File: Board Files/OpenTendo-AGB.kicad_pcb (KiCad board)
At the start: 2 copper layers, 131.3 x 72.4 mm, 221 parts, among them P1 CART-SLOT, P2 LCD, U2 AGB-SRAM, U3 AGB-REG, X2 Crystal

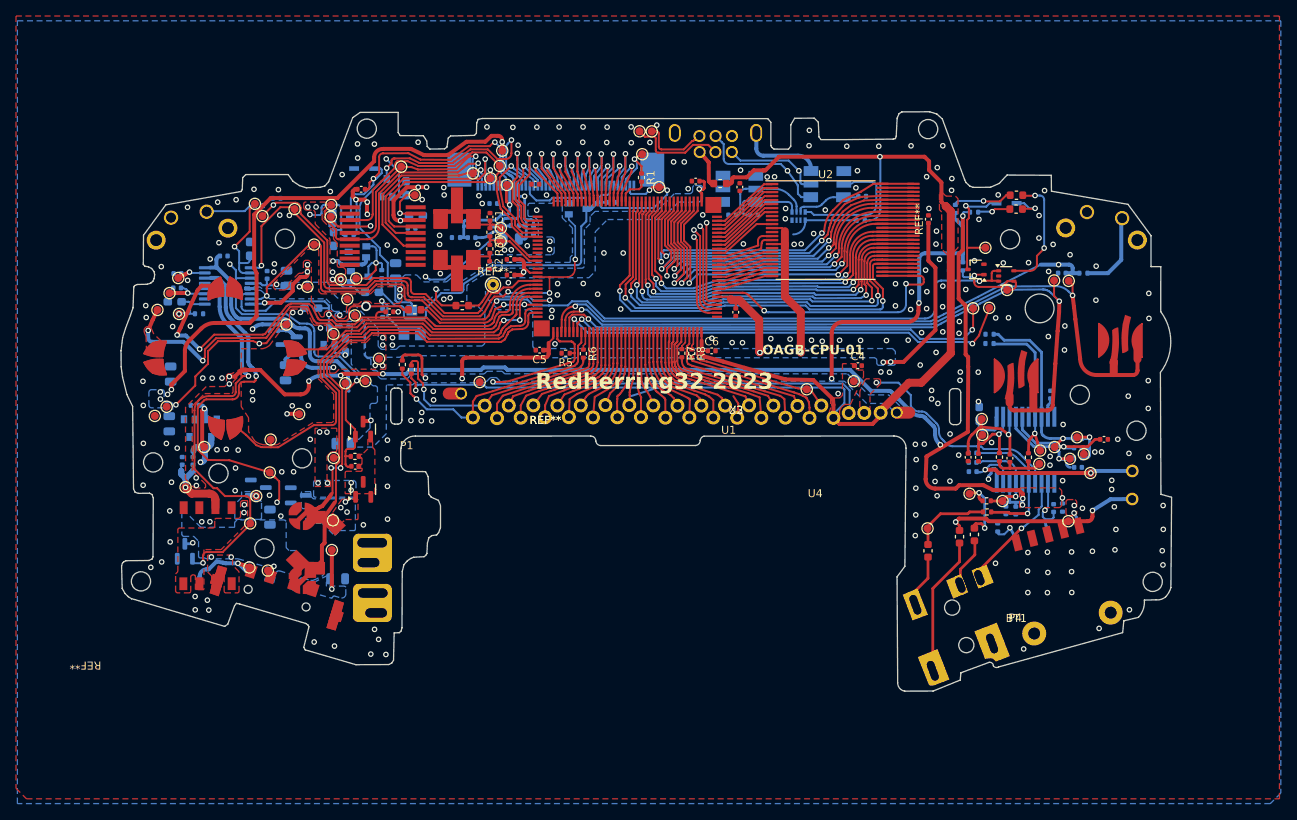
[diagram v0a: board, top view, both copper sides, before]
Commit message: Add files via upload
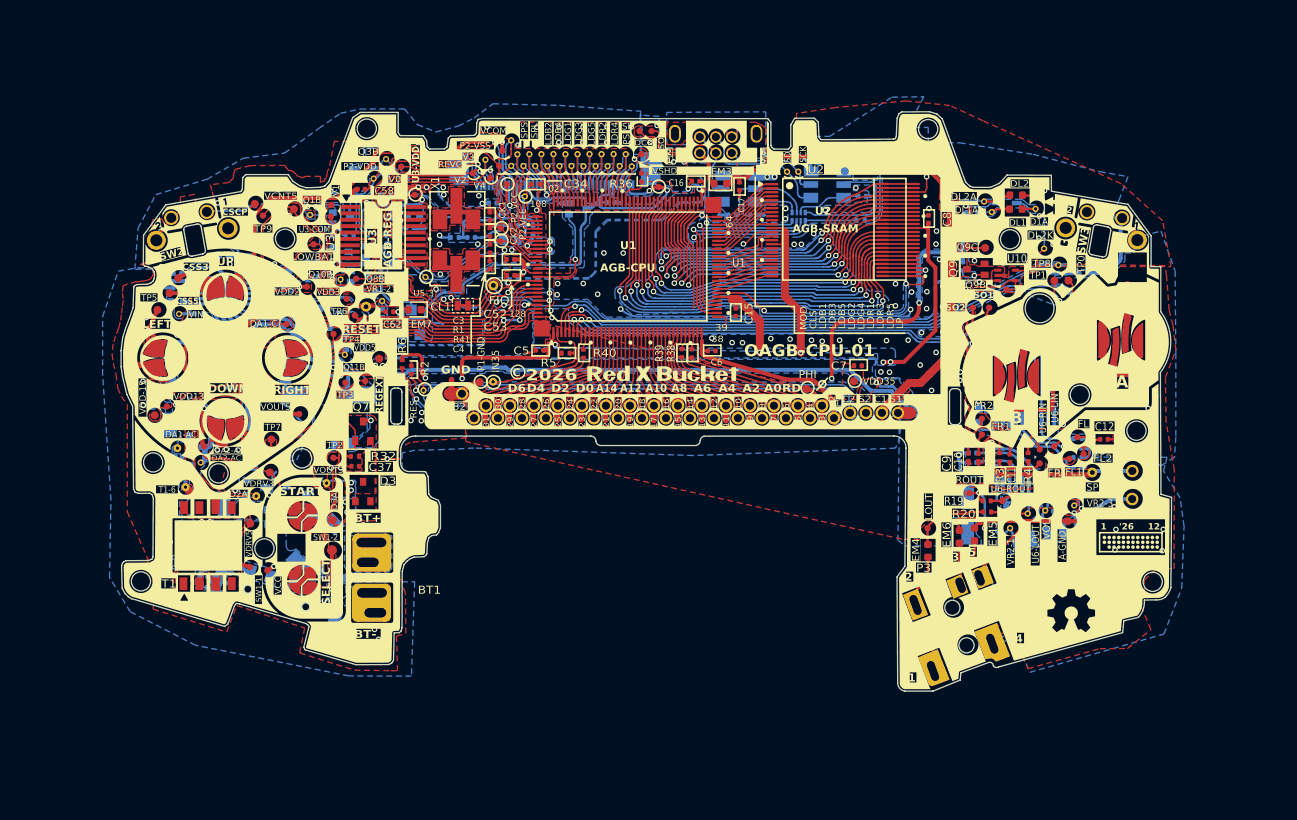
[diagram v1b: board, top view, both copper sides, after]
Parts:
- removed  : SOT-23-Small, OpenTendo-AGB:SOT-23-Small
- removed  : LR, OpenTendo-AGB:LR
- removed  : R_0402_1005Metric, Resistor_SMD:R_0402_1005Metric
- removed  : TestPoint_Pad_D1.0mm, TestPoint:TestPoint_Pad_D1.0mm (x3)
- removed the C1 at (45.9, -59.6)
- removed the C2 at (45.9, -53.6)
- removed the R3 at (45.9, -55.6)
- removed REF**: C_0603_1608Metric_Pad1.08x0.95mm_HandSolder, Capacitor_SMD:C_0603_1608Metric_Pad1.08x0.95mm_HandSolder
- removed REF** (x2): C_0402_1005Metric, Capacitor_SMD:C_0402_1005Metric
- added C13: 0.1u, OpenTendo-AGB:C_0402_1005Metric, B.Cu at (46.2, -61.4)
- added C3: 27p, OpenTendo-AGB:C_0402_1005Metric, F.Cu at (45.9, -59.7)
- added C4: 33p, OpenTendo-AGB:C_0402_1005Metric, F.Cu at (45.9, -53.6)
- added C42: 1u, OpenTendo-AGB:C_0603_1608Metric, B.Cu at (35.4, -63.5)
- added C49: 100p, OpenTendo-AGB:C_0402_1005Metric, B.Cu at (119.3, -28.3)
- added CP1: 100u, OpenTendo-AGB:CP_Elec_5x5.3, B.Cu at (12.7, -21.3)
- added CP2: 100u, OpenTendo-AGB:C_Elec_6.3x5.8, B.Cu at (16.1, -32.1)
- added CP3: 470u, OpenTendo-AGB:C_Elec_8x10.2, B.Cu at (25.9, -37.4)
- added CP4: 100u, OpenTendo-AGB:CP_Elec_5x5.3, B.Cu at (105.6, -22.4)
- added G***: LOGO, LOGO, F.Cu at (67.6, -40.1)
- added G***: LOGO, LOGO, F.Cu at (118.5, -10.4)
- added Q3: DTC114Y, OpenTendo-AGB:SOT-323, B.Cu at (32.9, -63.6)
- added R4: 47k, OpenTendo-AGB:R_0402_1005Metric, F.Cu at (113.2, -29.6)
- added R41: 2.2k, OpenTendo-AGB:R_0402_1005Metric, F.Cu at (45.9, -55.7)
- added SW2: SW_Push, OpenTendo-AGB:L, F.Cu at (10.5, -60.3)
- added TP0: TP0, OpenTendo-AGB:TestPoint_Pad_D1.0mm, F.Cu at (118.2, -51.7)
- added TP10: VOUT3, OpenTendo-AGB:TestPoint_Pad_D1.0mm_VIA, F.Cu at (25.5, -26.4)
- added TP106: VOL, OpenTendo-AGB:TestPoint_Pad_D0.8mm_VIA, F.Cu at (115.3, -22.9)
- added TP107: VR2-3, OpenTendo-AGB:TestPoint_Pad_D0.8mm_VIA, F.Cu at (118.9, -23.6)
- added TP108: VR2-1, OpenTendo-AGB:TestPoint_Pad_D0.8mm_VIA, F.Cu at (110.9, -20.7)
- added TP109: LOUT, OpenTendo-AGB:TestPoint_Pad_D0.8mm, F.Cu at (100.6, -20.7)
- added TP111: SP, OpenTendo-AGB:TestPoint_Pad_D1.25mm_VIA, F.Cu at (121.2, -27.7)
- added TP15: ~{RESET}, OpenTendo-AGB:TestPoint_Pad_D1.25mm_VIA, F.Cu at (30.4, -48.4)
- added TP18: DA2-AC, OpenTendo-AGB:TestPoint_Pad_D0.8mm_VIA, F.Cu at (9.74, -28.9)
- added TP19: DA1-AC, OpenTendo-AGB:TestPoint_Pad_D1.0mm_VIA, F.Cu at (6.83, -30.8)
- added TP28: LOWBAT, OpenTendo-AGB:TestPoint_Pad_D0.8mm, F.Cu at (23.9, -56.2)
- added TP29: DL2A, OpenTendo-AGB:TestPoint_Pad_D0.8mm_VIA, F.Cu at (107.7, -61.6)
- added TP30: DL2K, OpenTendo-AGB:TestPoint_Pad_D0.8mm_VIA, F.Cu at (115.2, -55.7)
- added TP31: DL1A, OpenTendo-AGB:TestPoint_Pad_D0.8mm_VIA, F.Cu at (108.6, -60.3)
- added TP32: D1A, OpenTendo-AGB:TestPoint_Pad_D0.8mm_VIA, F.Cu at (114.1, -60.6)
- added TP35: Q11B, OpenTendo-AGB:TestPoint_Pad_D0.8mm_VIA, F.Cu at (27.8, -42.4)
- added TP36: MOD, OpenTendo-AGB:TestPoint_Pad_D0.8mm_VIA, F.Cu at (48.5, -66.0)
- added TP37: SPS, OpenTendo-AGB:TestPoint_Pad_D0.8mm_VIA, F.Cu at (49.3, -67.5)
- added TP38: CLS, OpenTendo-AGB:TestPoint_Pad_D0.8mm_VIA, F.Cu at (50.1, -66.0)
- added TP39: SPL, OpenTendo-AGB:TestPoint_Pad_D0.8mm_VIA, F.Cu at (50.8, -67.5)
- added TP40: LDB1, OpenTendo-AGB:TestPoint_Pad_D0.8mm_VIA, F.Cu at (51.6, -66.0)
- added TP41: LDB2, OpenTendo-AGB:TestPoint_Pad_D0.8mm_VIA, F.Cu at (52.3, -67.5)
- added TP42: LDB3, OpenTendo-AGB:TestPoint_Pad_D0.8mm_VIA, F.Cu at (53.1, -66.0)
- added TP43: LDB4, OpenTendo-AGB:TestPoint_Pad_D0.8mm_VIA, F.Cu at (53.8, -67.5)
- added TP44: LDB5, OpenTendo-AGB:TestPoint_Pad_D0.8mm_VIA, F.Cu at (54.6, -66.0)
- added TP45: LDG1, OpenTendo-AGB:TestPoint_Pad_D0.8mm_VIA, F.Cu at (55.3, -67.5)
- added TP46: LDG2, OpenTendo-AGB:TestPoint_Pad_D0.8mm_VIA, F.Cu at (56.1, -66.0)
- added TP47: LDG3, OpenTendo-AGB:TestPoint_Pad_D0.8mm_VIA, F.Cu at (56.8, -67.5)
- added TP48: LDG4, OpenTendo-AGB:TestPoint_Pad_D0.8mm_VIA, F.Cu at (57.6, -66.0)
- added TP49: LDG5, OpenTendo-AGB:TestPoint_Pad_D0.8mm_VIA, F.Cu at (58.3, -67.5)
- added TP50: LDR1, OpenTendo-AGB:TestPoint_Pad_D0.8mm_VIA, F.Cu at (59.1, -66.0)
- added TP51: LDR2, OpenTendo-AGB:TestPoint_Pad_D0.8mm_VIA, F.Cu at (59.8, -67.5)
- added TP52: LDR3, OpenTendo-AGB:TestPoint_Pad_D0.8mm_VIA, F.Cu at (60.6, -66.0)
- added TP53: LDR4, OpenTendo-AGB:TestPoint_Pad_D0.8mm_VIA, F.Cu at (61.4, -67.5)
- added TP54: LDR5, OpenTendo-AGB:TestPoint_Pad_D0.8mm_VIA, F.Cu at (62.1, -66.0)
- added TP55: PS, OpenTendo-AGB:TestPoint_Pad_D0.8mm_VIA, F.Cu at (62.9, -67.5)
- added TP56: LP, OpenTendo-AGB:TestPoint_Pad_D0.8mm_VIA, F.Cu at (63.6, -66.0)
- added TP60: P2-VDD, OpenTendo-AGB:TestPoint_Pad_D0.8mm_VIA, F.Cu at (31.4, -64.4)
- added TP61: P2-VEE, OpenTendo-AGB:TestPoint_Pad_D0.8mm_VIA, F.Cu at (50.2, -62.2)
- added TP67: V3, OpenTendo-AGB:TestPoint_Pad_D0.8mm_VIA, F.Cu at (45.3, -66.8)
- added TP70: VCOM, OpenTendo-AGB:TestPoint_Pad_D0.8mm_VIA, F.Cu at (48.5, -69.2)
- added TP71: VR1-2, OpenTendo-AGB:TestPoint_Pad_D0.8mm_VIA, F.Cu at (32.4, -49.1)
- added TP72: U5-3, OpenTendo-AGB:TestPoint_Pad_D0.8mm_VIA, F.Cu at (37.8, -52.1)
- added TP73: Q3B, OpenTendo-AGB:TestPoint_Pad_D0.8mm_VIA, F.Cu at (32.9, -66.9)
- added TP74: Q1B, OpenTendo-AGB:TestPoint_Pad_D0.8mm_VIA, F.Cu at (23.4, -59.9)
- added TP75: IN35, OpenTendo-AGB:TestPoint_Pad_D1.0mm_VIA, F.Cu at (46.3, -39.0)
- added TP78: RES, OpenTendo-AGB:TestPoint_Pad_D0.8mm_VIA, F.Cu at (37.6, -38.0)
- added TP8: TP8, OpenTendo-AGB:TestPoint_Pad_D0.8mm_VIA, F.Cu at (116.9, -53.6)
- added TP93: SD, OpenTendo-AGB:TestPoint_Pad_D0.8mm_VIA, F.Cu at (83.0, -65.3)
- added TP95: SCK, OpenTendo-AGB:TestPoint_Pad_D0.8mm_VIA, F.Cu at (84.4, -65.3)
- added U5: ~, OpenTendo-AGB:SOT-363_SC-70-6, B.Cu at (32.9, -58.5)
- C1, C63, C64: renamed from REF**; value C_0402_1005Metric -> 0.01u; footprint Capacitor_SMD:C_0402_1005Metric -> OpenTendo-AGB:C_0402_1005Metric
- C10: renamed from  ; value C_0402_1005Metric -> 100p; footprint Capacitor_SMD:C_0402_1005Metric -> OpenTendo-AGB:C_0402_1005Metric
- C11: renamed from  ; value C_0402_1005Metric -> 470p; footprint Capacitor_SMD:C_0402_1005Metric -> OpenTendo-AGB:C_0402_1005Metric
- C12, C9: renamed from  ; value C_0402_1005Metric -> 1000p; footprint Capacitor_SMD:C_0402_1005Metric -> OpenTendo-AGB:C_0402_1005Metric
- C14, C22, C23, C26, C32, C39, C40, C41, C45, C46, C47, C50, C51, C55, C59, C8: renamed from REF**; value C_0402_1005Metric -> 0.1u; footprint Capacitor_SMD:C_0402_1005Metric -> OpenTendo-AGB:C_0402_1005Metric
- C15, C16, C17, C34, C52, C53, C58: renamed from  ; value C_0402_1005Metric -> 0.1u; footprint Capacitor_SMD:C_0402_1005Metric -> OpenTendo-AGB:C_0402_1005Metric
- C18, C19, C20: renamed from REF**; value C_0402_1005Metric -> 100p; footprint Capacitor_SMD:C_0402_1005Metric -> OpenTendo-AGB:C_0402_1005Metric
- C2, C24, C28, C30, C38, C57, C61: renamed from REF**; value C_0603_1608Metric_Pad1.08x0.95mm_HandSolder -> 1u; footprint Capacitor_SMD:C_0603_1608Metric_Pad1.08x0.95mm_HandSolder -> OpenTendo-AGB:C_0603_1608Metric
- C25: renamed from REF**; value C_0603_1608Metric_Pad1.08x0.95mm_HandSolder -> 0.47u; footprint Capacitor_SMD:C_0603_1608Metric_Pad1.08x0.95mm_HandSolder -> OpenTendo-AGB:C_0603_1608Metric
- C27, C43, C54: renamed from REF**; value C_0805_2012Metric -> 4.7u; footprint Capacitor_SMD:C_0805_2012Metric -> OpenTendo-AGB:C_0805_2012Metric
- C33, C35, C36: renamed from REF**; value C_0805_2012Metric -> 1u; footprint Capacitor_SMD:C_0805_2012Metric -> OpenTendo-AGB:C_0805_2012Metric
- C37, C62: renamed from  ; value C_0402_1005Metric -> 0.01u; footprint Capacitor_SMD:C_0402_1005Metric -> OpenTendo-AGB:C_0402_1005Metric
- C44, C56: renamed from REF**; value C_0805_2012Metric -> 2.2u; footprint Capacitor_SMD:C_0805_2012Metric -> OpenTendo-AGB:C_0805_2012Metric
- C48: renamed from REF**; value C_0402_1005Metric -> 470p; footprint Capacitor_SMD:C_0402_1005Metric -> OpenTendo-AGB:C_0402_1005Metric
- C5, C6: value C_Small -> 0.1u; footprint Capacitor_SMD:C_0402_1005Metric -> OpenTendo-AGB:C_0402_1005Metric
- C7: renamed from C4; value C_Small -> 0.1u; footprint Capacitor_SMD:C_0402_1005Metric -> OpenTendo-AGB:C_0402_1005Metric
- CL1: renamed from  ; value L_0603_1608Metric -> SolderJumper_2_Bridged; footprint Inductor_SMD:L_0603_1608Metric -> OpenTendo-AGB:Jumper-Bridged
- D1: renamed from REF**; value Diode -> MA112
- D2: renamed from  ; value SOT-23 -> RB411D; footprint Package_TO_SOT_SMD:SOT-23 -> OpenTendo-AGB:SOT-23
- D3: renamed from  ; value SOT-23 -> RB491D; footprint Package_TO_SOT_SMD:SOT-23 -> OpenTendo-AGB:SOT-23
- D4: renamed from REF**; value Diode -> ISS355
- DA1, DA2: renamed from  ; value SOT-23-Small -> DA204U; footprint OpenTendo-AGB:SOT-23-Small -> OpenTendo-AGB:SOT-323
- DL1: renamed from  ; value L_0603_1608Metric -> SML311UT; footprint Inductor_SMD:L_0603_1608Metric -> OpenTendo-AGB:LED_0603_1608Metric
- DL2: renamed from  ; value L_0603_1608Metric -> SML210MT; footprint Inductor_SMD:L_0603_1608Metric -> OpenTendo-AGB:LED_0603_1608Metric
- DZ1: renamed from REF**; value Diode -> 4.7V
- EM1, EM2: renamed from REF**; value EM -> ACM4532-102-3P
- EM3, EM4, EM5, EM6, EM7: renamed from  ; value L_0603_1608Metric -> L_Small; footprint Inductor_SMD:L_0603_1608Metric -> OpenTendo-AGB:L_0603_1608Metric
- F1: renamed from REF**; value Fuse_0805_2012Metric -> 4341.25; footprint Fuse:Fuse_0805_2012Metric -> OpenTendo-AGB:Fuse_0603_1608Metric
- L1: renamed from REF**; value Inductor -> 100u; moved to B.Cu
- P1: value CART-SLOT -> ~
- P2: value LCD -> ~
- P3: renamed from  ; value Audio-Jack -> PHONE JACK
- P4: value ~ -> AGB-LINK
- Q1: renamed from  ; value SOT-23-Small -> DTA123J; footprint OpenTendo-AGB:SOT-23-Small -> OpenTendo-AGB:SOT-323
- Q10: renamed from  ; value SOT-23-Small -> DTC114Y; footprint OpenTendo-AGB:SOT-23-Small -> OpenTendo-AGB:SOT-323
- Q11: renamed from  ; value SOT-23-Small -> DTA114Y; footprint OpenTendo-AGB:SOT-23-Small -> OpenTendo-AGB:SOT-323
- Q2: renamed from  ; value SOT-23-Small -> DTA114T; footprint OpenTendo-AGB:SOT-23-Small -> OpenTendo-AGB:SOT-323
- Q4, Q5: renamed from  ; value SOT-23 -> FDV303N; footprint Package_TO_SOT_SMD:SOT-23 -> OpenTendo-AGB:SOT-23
- Q6: renamed from  ; value SOT-23 -> 2SK1582; footprint Package_TO_SOT_SMD:SOT-23 -> OpenTendo-AGB:SOT-23
- Q7: renamed from  ; value SOT-23 -> SSM3J01F; footprint Package_TO_SOT_SMD:SOT-23 -> OpenTendo-AGB:SOT-23
- Q8: renamed from  ; value SOT-23-Small -> 2SC4081; footprint OpenTendo-AGB:SOT-23-Small -> OpenTendo-AGB:SOT-323
- Q9: renamed from  ; value SOT-323_SC-70 -> 2SC4081; footprint Package_TO_SOT_SMD:SOT-323_SC-70 -> OpenTendo-AGB:SOT-323
- R1: renamed from R2; value R_Small -> 1.5M; footprint Resistor_SMD:R_0402_1005Metric -> OpenTendo-AGB:R_0402_1005Metric
- R10, R37: renamed from REF**; value R_0402_1005Metric -> 470; footprint Resistor_SMD:R_0402_1005Metric -> OpenTendo-AGB:R_0402_1005Metric
- R11, R12, R13: renamed from REF**; value R_0402_1005Metric -> 150; footprint Resistor_SMD:R_0402_1005Metric -> OpenTendo-AGB:R_0402_1005Metric
- R14: renamed from REF**; value R_0402_1005Metric -> 4.7k; footprint Resistor_SMD:R_0402_1005Metric -> OpenTendo-AGB:R_0402_1005Metric
- R15, R16, R18: renamed from REF**; value R_0402_1005Metric -> 33k; footprint Resistor_SMD:R_0402_1005Metric -> OpenTendo-AGB:R_0402_1005Metric
- R17, R35: renamed from REF**; value R_0402_1005Metric -> 100k; footprint Resistor_SMD:R_0402_1005Metric -> OpenTendo-AGB:R_0402_1005Metric
- R19, R20: renamed from  ; value R_0402_1005Metric -> 15; footprint Resistor_SMD:R_0402_1005Metric -> OpenTendo-AGB:R_0402_1005Metric
- R2: renamed from  ; value R_0402_1005Metric -> 10k; footprint Resistor_SMD:R_0402_1005Metric -> OpenTendo-AGB:R_0402_1005Metric
- R25: renamed from REF**; value R_0402_1005Metric -> 47; footprint Resistor_SMD:R_0402_1005Metric -> OpenTendo-AGB:R_0402_1005Metric
- R26, R34: renamed from REF**; value R_0402_1005Metric -> 15k; footprint Resistor_SMD:R_0402_1005Metric -> OpenTendo-AGB:R_0402_1005Metric
- R27: renamed from REF**; value R_0402_1005Metric -> 200k; footprint Resistor_SMD:R_0402_1005Metric -> OpenTendo-AGB:R_0402_1005Metric
- R28: renamed from REF**; value R_0402_1005Metric -> 56k; footprint Resistor_SMD:R_0402_1005Metric -> OpenTendo-AGB:R_0402_1005Metric
- R29: renamed from REF**; value R_0402_1005Metric -> 18k; footprint Resistor_SMD:R_0402_1005Metric -> OpenTendo-AGB:R_0402_1005Metric
- R3: renamed from  ; value R_0402_1005Metric -> 47k; footprint Resistor_SMD:R_0402_1005Metric -> OpenTendo-AGB:R_0402_1005Metric
- R30, R31, R7, R8: renamed from REF**; value R_0402_1005Metric -> 47k; footprint Resistor_SMD:R_0402_1005Metric -> OpenTendo-AGB:R_0402_1005Metric
- R32: renamed from  ; value R_0402_1005Metric -> 1M; footprint Resistor_SMD:R_0402_1005Metric -> OpenTendo-AGB:R_0402_1005Metric
- R33: renamed from REF**; value R_0402_1005Metric -> 5.1; footprint Resistor_SMD:R_0402_1005Metric -> OpenTendo-AGB:R_0402_1005Metric
- R36: renamed from R1; value R_Small -> 270; footprint Resistor_SMD:R_0402_1005Metric -> OpenTendo-AGB:R_0402_1005Metric
- R38: renamed from R8; value R_Small -> 47; footprint Resistor_SMD:R_0402_1005Metric -> OpenTendo-AGB:R_0402_1005Metric
- R39: renamed from R7; value R_Small -> 47; footprint Resistor_SMD:R_0402_1005Metric -> OpenTendo-AGB:R_0402_1005Metric
- R40: renamed from R6; value R_Small -> 15; footprint Resistor_SMD:R_0402_1005Metric -> OpenTendo-AGB:R_0402_1005Metric
- R43, R44: renamed from REF**; value R_0402_1005Metric -> 15; footprint Resistor_SMD:R_0402_1005Metric -> OpenTendo-AGB:R_0402_1005Metric
- R5: value R_Small -> 100k; footprint Resistor_SMD:R_0402_1005Metric -> OpenTendo-AGB:R_0402_1005Metric
- R6: renamed from  ; value R_0402_1005Metric -> 100k; footprint Resistor_SMD:R_0402_1005Metric -> OpenTendo-AGB:R_0402_1005Metric
- RA1: renamed from REF**; value RA -> 330
- SP1: renamed from  
- SW1: renamed from REF**; value Power Switch -> AGB-SW; moved to B.Cu
- SW3: renamed from  ; value R -> SW_Push
- SW4: renamed from  ; value AB -> ~
- SW5: renamed from  ; value StartSelect -> ~
- T1: renamed from  ; value Coil -> AGB-XFRM
- TP1: renamed from  ; value TestPoint_Pad_D1.0mm -> TP1; footprint TestPoint:TestPoint_Pad_D1.0mm -> OpenTendo-AGB:TestPoint_Pad_D1.0mm
- TP100: renamed from  ; value TestPoint_Pad_D1.0mm -> FL1; footprint TestPoint:TestPoint_Pad_D1.0mm -> OpenTendo-AGB:TestPoint_Pad_D0.8mm
- TP101: renamed from  ; value TestPoint_Pad_D1.0mm -> FL2; footprint TestPoint:TestPoint_Pad_D1.0mm -> OpenTendo-AGB:TestPoint_Pad_D0.8mm
- TP102: renamed from  ; value TestPoint_Pad_D1.0mm -> FR1; footprint TestPoint:TestPoint_Pad_D1.0mm -> OpenTendo-AGB:TestPoint_Pad_D0.8mm
- TP103: renamed from  ; value TestPoint_Pad_D1.0mm -> FR2; footprint TestPoint:TestPoint_Pad_D1.0mm -> OpenTendo-AGB:TestPoint_Pad_D0.8mm
- TP104: renamed from  ; value TestPoint_Pad_D1.0mm -> U6-LOUT; footprint TestPoint:TestPoint_Pad_D1.0mm -> OpenTendo-AGB:TestPoint_Pad_D0.8mm_VIA
- TP105: renamed from  ; value TestPoint_Pad_D1.0mm -> U6-ROUT; footprint TestPoint:TestPoint_Pad_D1.0mm -> OpenTendo-AGB:TestPoint_Pad_D0.8mm
- TP11: renamed from  ; value TestPoint_Pad_D1.0mm -> VDRV3; footprint TestPoint:TestPoint_Pad_D1.0mm -> OpenTendo-AGB:TestPoint_Pad_D1.0mm
- TP110: renamed from  ; value TestPoint_Pad_D1.0mm -> ROUT; footprint TestPoint:TestPoint_Pad_D1.0mm -> OpenTendo-AGB:TestPoint_Pad_D0.8mm
- TP112: renamed from  ; value TestPoint_Pad_D1.0mm -> A-GND; footprint TestPoint:TestPoint_Pad_D1.0mm -> OpenTendo-AGB:TestPoint_Pad_D1.0mm
- TP113: renamed from  ; value TestPoint_Pad_D1.0mm -> VDD3; footprint TestPoint:TestPoint_Pad_D1.0mm -> OpenTendo-AGB:TestPoint_Pad_D0.8mm
- TP114: renamed from  ; value TestPoint_Pad_D1.0mm -> R-OUT; footprint TestPoint:TestPoint_Pad_D1.0mm -> OpenTendo-AGB:TestPoint_Pad_D0.8mm
- TP115: renamed from  ; value TestPoint_Pad_D1.0mm -> L-OUT; footprint TestPoint:TestPoint_Pad_D1.0mm -> OpenTendo-AGB:TestPoint_Pad_D0.8mm
- TP116: renamed from  ; value TestPoint_Pad_D1.0mm -> T1-6; footprint TestPoint:TestPoint_Pad_D1.0mm -> OpenTendo-AGB:TestPoint_Pad_D1.0mm_VIA
- TP12: renamed from  ; value TestPoint_Pad_D1.0mm -> VDD2; footprint TestPoint:TestPoint_Pad_D1.0mm -> OpenTendo-AGB:TestPoint_Pad_D0.8mm
- TP13: renamed from  ; value TestPoint_Pad_D1.0mm -> VDRV5; footprint TestPoint:TestPoint_Pad_D1.0mm -> OpenTendo-AGB:TestPoint_Pad_D1.0mm
- TP14: renamed from  ; value TestPoint_Pad_D1.0mm -> VOUT5; footprint TestPoint:TestPoint_Pad_D1.0mm -> OpenTendo-AGB:TestPoint_Pad_D0.8mm
- TP16: renamed from  ; value TestPoint_Pad_D1.0mm -> D3A; footprint TestPoint:TestPoint_Pad_D1.0mm -> OpenTendo-AGB:TestPoint_Pad_D1.0mm
- TP17: renamed from  ; value TestPoint_Pad_D1.0mm -> D2A; footprint TestPoint:TestPoint_Pad_D1.0mm -> OpenTendo-AGB:TestPoint_Pad_D1.0mm_VIA
- TP2: renamed from  ; value TestPoint_Pad_D1.0mm -> TP2; footprint TestPoint:TestPoint_Pad_D1.0mm -> OpenTendo-AGB:TestPoint_Pad_D0.8mm
- TP20: renamed from  ; value TestPoint_Pad_D1.0mm -> DA2-A; footprint TestPoint:TestPoint_Pad_D1.0mm -> OpenTendo-AGB:TestPoint_Pad_D0.8mm
- TP21: renamed from  ; value TestPoint_Pad_D1.0mm -> DA1-C; footprint TestPoint:TestPoint_Pad_D1.0mm -> OpenTendo-AGB:TestPoint_Pad_D0.8mm
- TP22: renamed from  ; value TestPoint_Pad_D1.0mm -> VDD13; footprint TestPoint:TestPoint_Pad_D1.0mm -> OpenTendo-AGB:TestPoint_Pad_D0.8mm
- TP23: renamed from  ; value TestPoint_Pad_D1.0mm -> VDD-15; footprint TestPoint:TestPoint_Pad_D1.0mm -> OpenTendo-AGB:TestPoint_Pad_D1.0mm
- TP24: renamed from  ; value TestPoint_Pad_D1.0mm -> VDD5; footprint TestPoint:TestPoint_Pad_D1.0mm -> OpenTendo-AGB:TestPoint_Pad_D1.0mm
- TP25: renamed from  ; value TestPoint_Pad_D1.0mm -> Q8B; footprint TestPoint:TestPoint_Pad_D1.0mm -> OpenTendo-AGB:TestPoint_Pad_D0.8mm
- TP26: renamed from  ; value TestPoint_Pad_D1.0mm -> VSHD; footprint TestPoint:TestPoint_Pad_D1.0mm -> OpenTendo-AGB:TestPoint_Pad_D0.8mm
- TP27: renamed from  ; value TestPoint_Pad_D1.0mm -> Q10B; footprint TestPoint:TestPoint_Pad_D1.0mm -> OpenTendo-AGB:TestPoint_Pad_D0.8mm_VIA
- TP3: renamed from  ; value TestPoint_Pad_D1.0mm -> TP3; footprint TestPoint:TestPoint_Pad_D1.0mm -> OpenTendo-AGB:TestPoint_Pad_D0.8mm
- TP33: renamed from  ; value TestPoint_Pad_D1.0mm -> Q9C; footprint TestPoint:TestPoint_Pad_D1.0mm -> OpenTendo-AGB:TestPoint_Pad_D1.0mm
- TP34: renamed from  ; value TestPoint_Pad_D1.0mm -> Q9B; footprint TestPoint:TestPoint_Pad_D1.0mm -> OpenTendo-AGB:TestPoint_Pad_D0.8mm
- TP4: renamed from  ; value TestPoint_Pad_D1.0mm -> TP4; footprint TestPoint:TestPoint_Pad_D1.0mm -> OpenTendo-AGB:TestPoint_Pad_D0.8mm
- TP5: renamed from  ; value TestPoint_Pad_D1.0mm -> TP5; footprint TestPoint:TestPoint_Pad_D1.0mm -> OpenTendo-AGB:TestPoint_Pad_D1.0mm
- TP57: renamed from  ; value TestPoint_Pad_D1.0mm -> DCK; footprint TestPoint:TestPoint_Pad_D1.0mm -> OpenTendo-AGB:TestPoint_Pad_D0.8mm
- TP58: renamed from  ; value TestPoint_Pad_D1.0mm -> P2-VSS; footprint TestPoint:TestPoint_Pad_D1.0mm -> OpenTendo-AGB:TestPoint_Pad_D0.8mm
- TP59: renamed from  ; value TestPoint_Pad_D1.0mm -> P2-VCC; footprint TestPoint:TestPoint_Pad_D1.0mm -> OpenTendo-AGB:TestPoint_Pad_D0.8mm
- TP6: renamed from  ; value TestPoint_Pad_D1.0mm -> TP6; footprint TestPoint:TestPoint_Pad_D1.0mm -> OpenTendo-AGB:TestPoint_Pad_D0.8mm
- TP62: renamed from  ; value TestPoint_Pad_D1.0mm -> REVC; footprint TestPoint:TestPoint_Pad_D1.0mm -> OpenTendo-AGB:TestPoint_Pad_D0.8mm
- TP63: renamed from  ; value TestPoint_Pad_D1.0mm -> U3-VDD; footprint TestPoint:TestPoint_Pad_D1.0mm -> OpenTendo-AGB:TestPoint_Pad_D0.8mm
- TP64: renamed from  ; value TestPoint_Pad_D1.0mm -> V0; footprint TestPoint:TestPoint_Pad_D1.0mm -> OpenTendo-AGB:TestPoint_Pad_D0.8mm
- TP65: renamed from  ; value TestPoint_Pad_D1.0mm -> V1; footprint TestPoint:TestPoint_Pad_D1.0mm -> OpenTendo-AGB:TestPoint_Pad_D0.8mm
- TP66: renamed from  ; value TestPoint_Pad_D1.0mm -> V2; footprint TestPoint:TestPoint_Pad_D1.0mm -> OpenTendo-AGB:TestPoint_Pad_D0.8mm
- TP68: renamed from  ; value TestPoint_Pad_D1.0mm -> V4; footprint TestPoint:TestPoint_Pad_D1.0mm -> OpenTendo-AGB:TestPoint_Pad_D0.8mm
- TP69: renamed from  ; value TestPoint_Pad_D1.0mm -> U3-COM; footprint TestPoint:TestPoint_Pad_D1.0mm -> OpenTendo-AGB:TestPoint_Pad_D0.8mm
- TP7: renamed from  ; value TestPoint_Pad_D1.0mm -> TP7; footprint TestPoint:TestPoint_Pad_D1.0mm -> OpenTendo-AGB:TestPoint_Pad_D1.0mm
- TP76: renamed from  ; value TestPoint_Pad_D1.0mm -> VDD35; footprint TestPoint:TestPoint_Pad_D1.0mm -> OpenTendo-AGB:TestPoint_Pad_D1.0mm
- TP77: renamed from  ; value TestPoint_Pad_D1.0mm -> PHI; footprint TestPoint:TestPoint_Pad_D1.0mm -> OpenTendo-AGB:TestPoint_Pad_D1.0mm
- TP79: renamed from  ; value TestPoint_Pad_D1.0mm -> P1-GND; footprint TestPoint:TestPoint_Pad_D1.0mm -> OpenTendo-AGB:TestPoint_Pad_D1.0mm
- TP80: renamed from  ; value TestPoint_Pad_D1.0mm -> CK1; footprint TestPoint:TestPoint_Pad_D1.0mm -> OpenTendo-AGB:TestPoint_Pad_D0.8mm
- TP81: renamed from  ; value TestPoint_Pad_D1.0mm -> CK2; footprint TestPoint:TestPoint_Pad_D1.0mm -> OpenTendo-AGB:TestPoint_Pad_D0.8mm
- TP82: renamed from REF**; value TestPoint_THTPad_D1.5mm_Drill0.7mm -> FIQ; footprint TestPoint:TestPoint_THTPad_D1.5mm_Drill0.7mm -> OpenTendo-AGB:TestPoint_Pad_D1.25mm_VIA
- TP83: renamed from  ; value TestPoint_Pad_D1.0mm -> SW1-2; footprint TestPoint:TestPoint_Pad_D1.0mm -> OpenTendo-AGB:TestPoint_Pad_D1.25mm
- TP84: renamed from  ; value TestPoint_Pad_D1.0mm -> SW1-1; footprint TestPoint:TestPoint_Pad_D1.0mm -> OpenTendo-AGB:TestPoint_Pad_D0.8mm
- TP85: renamed from  ; value TestPoint_Pad_D1.0mm -> VCC; footprint TestPoint:TestPoint_Pad_D1.0mm -> OpenTendo-AGB:TestPoint_Pad_D0.8mm
- TP86: renamed from  ; value TestPoint_Pad_D1.0mm -> C_SCP; footprint TestPoint:TestPoint_Pad_D1.0mm -> OpenTendo-AGB:TestPoint_Pad_D1.0mm
- TP87: renamed from  ; value TestPoint_Pad_D1.0mm -> C_SS5; footprint TestPoint:TestPoint_Pad_D1.0mm -> OpenTendo-AGB:TestPoint_Pad_D1.0mm
- TP88: renamed from  ; value TestPoint_Pad_D1.0mm -> C_SS3; footprint TestPoint:TestPoint_Pad_D1.0mm -> OpenTendo-AGB:TestPoint_Pad_D1.0mm
- TP89: renamed from  ; value TestPoint_Pad_D1.0mm -> VIN; footprint TestPoint:TestPoint_Pad_D1.0mm -> OpenTendo-AGB:TestPoint_Pad_D0.8mm_VIA
- TP9: renamed from  ; value TestPoint_Pad_D1.0mm -> TP9; footprint TestPoint:TestPoint_Pad_D1.0mm -> OpenTendo-AGB:TestPoint_Pad_D0.8mm
- TP90: renamed from  ; value TestPoint_Pad_D1.0mm -> REG_EXT; footprint TestPoint:TestPoint_Pad_D1.0mm -> OpenTendo-AGB:TestPoint_Pad_D0.8mm
- TP91: renamed from  ; value TestPoint_Pad_D1.0mm -> VCNT5; footprint TestPoint:TestPoint_Pad_D1.0mm -> OpenTendo-AGB:TestPoint_Pad_D1.0mm
- TP92: renamed from  ; value TestPoint_Pad_D1.0mm -> SO; footprint TestPoint:TestPoint_Pad_D1.0mm -> OpenTendo-AGB:TestPoint_Pad_D0.8mm
- TP94: renamed from  ; value TestPoint_Pad_D1.0mm -> SI; footprint TestPoint:TestPoint_Pad_D1.0mm -> OpenTendo-AGB:TestPoint_Pad_D0.8mm
- TP96: renamed from  ; value TestPoint_Pad_D1.0mm -> U6-LIN; footprint TestPoint:TestPoint_Pad_D1.0mm -> OpenTendo-AGB:TestPoint_Pad_D0.8mm
- TP97: renamed from  ; value TestPoint_Pad_D1.0mm -> U6-RIN; footprint TestPoint:TestPoint_Pad_D1.0mm -> OpenTendo-AGB:TestPoint_Pad_D0.8mm
- TP98: renamed from  ; value TestPoint_Pad_D1.0mm -> FL; footprint TestPoint:TestPoint_Pad_D1.0mm -> OpenTendo-AGB:TestPoint_Pad_D0.8mm
- TP99: renamed from  ; value TestPoint_Pad_D1.0mm -> FR; footprint TestPoint:TestPoint_Pad_D1.0mm -> OpenTendo-AGB:TestPoint_Pad_D0.8mm
- U1: value ~ -> AGB-CPU
- U10: renamed from  ; value SOT-353_SC-70-5 -> ~; footprint Package_TO_SOT_SMD:SOT-353_SC-70-5 -> OpenTendo-AGB:SOT-353_SC-70-5
- U2: value AGB-SRAM -> ~
- U4: renamed from REF**; value TSSOP-16_4.4x5mm_P0.65mm -> ~; footprint Package_SO:TSSOP-16_4.4x5mm_P0.65mm -> OpenTendo-AGB:TSSOP-16_4.4x5mm_P0.65mm
- U6: renamed from  ; value AGB-REG -> AGB-AMP; footprint OpenTendo-AGB:AGB-REG -> OpenTendo-AGB:AGB-AMP
- VR1: renamed from  ; value SOT-23-Large -> 50k; footprint OpenTendo-AGB:SOT-23-Large -> OpenTendo-AGB:VR1
- VR2: renamed from REF**; value Thumbwheel -> 30k; moved to B.Cu
- X1: renamed from X2; value Crystal -> 4.194304MHz
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- renumbered U4 to SW6
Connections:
- net /A renamed /CPU/TP0
- net /B renamed /CPU/TP1
- net /CART-A0 renamed /CPU/A_{0}
- net /CART-A1 renamed /CPU/A_{1}
- net /CART-A10 renamed /CPU/A_{10}
- net /CART-A11 renamed /CPU/A_{11}
- net /CART-A12 renamed /CPU/A_{12}
- net /CART-A13 renamed /CPU/A_{13}
- net /CART-A14 renamed /CPU/A_{14}
- net /CART-A15 renamed /CPU/A_{15}
- net /CART-A2 renamed /CPU/A_{2}
- net /CART-A3 renamed /CPU/A_{3}
- net /CART-A4 renamed /CPU/A_{4}
- net /CART-A5 renamed /CPU/A_{5}
- net /CART-A6 renamed /CPU/A_{6}
- net /CART-A7 renamed /CPU/A_{7}
- net /CART-A8 renamed /CPU/A_{8}
- net /CART-A9 renamed /CPU/A_{9}
- net /CART-D0 renamed /CPU/D_{0}
- net /CART-D1 renamed /CPU/D_{1}
- net /CART-D2 renamed /CPU/D_{2}
- net /CART-D3 renamed /CPU/D_{3}
- net /CART-D4 renamed /CPU/D_{4}
- net /CART-D5 renamed /CPU/D_{5}
- net /CART-D6 renamed /CPU/D_{6}
- net /CART-D7 renamed /CPU/D_{7}
- net /CLK1 renamed /CPU/CK1
- net /CLK2 renamed /CPU/CK2
- net /CLS renamed /CPU/CLS
- net /DCK renamed /CPU/DCK_{R}
- net /DOWN renamed /CPU/TP7
- net /IN35 renamed /CPU/IN35
- net /LDB1 renamed /CPU/LDB1
- net /LDB2 renamed /CPU/LDB2
- net /LDB3 renamed /CPU/LDB3
- net /LDB4 renamed /CPU/LDB4
- net /LDB5 renamed /CPU/LDB5
- net /LDG1 renamed /CPU/LDG1
- net /LDG2 renamed /CPU/LDG2
- net /LDG3 renamed /CPU/LDG3
- net /LDG4 renamed /CPU/LDG4
- net /LDG5 renamed /CPU/LDG5
- net /LDR1 renamed /CPU/LDR1
- net /LDR2 renamed /CPU/LDR2
- net /LDR3 renamed /CPU/LDR3
- net /LDR4 renamed /CPU/LDR4
- net /LDR5 renamed /CPU/LDR5
- net /LEFT renamed /CPU/TP5
- net /LP renamed /CPU/LP
- net /MOD renamed /CPU/MOD
- net /PHI renamed /CPU/PHI
- net /PS renamed /CPU/PS
- net /REVC renamed /CPU/REVC
- net /RIGHT renamed /CPU/TP4
- net /SELECT renamed /CPU/TP2
- net /SPL renamed /CPU/SPL
- net /SPS renamed /CPU/SPS
- net /SRAM-A0 renamed /CPU/MA_{0}
- net /SRAM-A1 renamed /CPU/MA_{1}
- net /SRAM-A10 renamed /CPU/MA_{10}
- net /SRAM-A11 renamed /CPU/MA_{11}
- net /SRAM-A12 renamed /CPU/MA_{12}
- net /SRAM-A13 renamed /CPU/MA_{13}
- net /SRAM-A14 renamed /CPU/MA_{14}
- net /SRAM-A15 renamed /CPU/MA_{15}
- net /SRAM-A16 renamed /CPU/MA_{16}
- net /SRAM-A2 renamed /CPU/MA_{2}
- net /SRAM-A3 renamed /CPU/MA_{3}
- net /SRAM-A4 renamed /CPU/MA_{4}
- net /SRAM-A5 renamed /CPU/MA_{5}
- net /SRAM-A6 renamed /CPU/MA_{6}
- net /SRAM-A8 renamed /CPU/MA_{8}
- net /SRAM-A9 renamed /CPU/MA_{9}
- net /SRAM-I/O1 renamed /CPU/MD_{0}
- net /SRAM-I/O10 renamed /CPU/MD_{9}
- net /SRAM-I/O11 renamed /CPU/MD_{10}
- net /SRAM-I/O12 renamed /CPU/MD_{11}
- net /SRAM-I/O13 renamed /CPU/MD_{12}
- net /SRAM-I/O14 renamed /CPU/MD_{13}
- net /SRAM-I/O15 renamed /CPU/MD_{14}
- net /SRAM-I/O16 renamed /CPU/MD_{15}
- net /SRAM-I/O2 renamed /CPU/MD_{1}
- net /SRAM-I/O3 renamed /CPU/MD_{2}
- net /SRAM-I/O4 renamed /CPU/MD_{3}
- net /SRAM-I/O5 renamed /CPU/MD_{4}
- net /SRAM-I/O6 renamed /CPU/MD_{5}
- net /SRAM-I/O7 renamed /CPU/MD_{6}
- net /SRAM-I/O8 renamed /CPU/MD_{7}
- net /SRAM-I/O9 renamed /CPU/MD_{8}
- net /SRAM-/LB renamed /CPU/~{LB}
- net /SRAM-/OE renamed /CPU/~{OE}_{RAM}
- net /SRAM-/UB renamed /CPU/~{UB}
- net /SRAM-/WE renamed /CPU/~{WE}_{RAM}
- net /START renamed /CPU/TP3
- net /V2 renamed /CPU/LCD/V2
- net /V3 renamed /CPU/LCD/V3
- net /V4 renamed /CPU/LCD/V4
- net //RD renamed /CPU/~{RD}
- net Net-(P2-DCK) renamed /CPU/LCD/DCK
- BT1 pad 1: /BAT+ -> /BT+
- C1 pad 1: (no net) -> VDD5
- C1 pad 2: (no net) -> GND
- C10 pad 1: (no net) -> /CPU/FR1
- C10 pad 2: (no net) -> GND
- C11 pad 1: (no net) -> /CPU/FR
- C11 pad 2: (no net) -> /CPU/FR2
- C12 pad 1: (no net) -> /CPU/FL2
- C12 pad 2: (no net) -> GND
- C14 pad 1: (no net) -> /VSHD
- C14 pad 2: /VSHD -> GND
- C15 pad 1: (no net) -> VDD2
- C15 pad 2: unconnected-(U1-VDD2-Pad44) -> GND
- C16 pad 1: /VDD2 -> VDD2
- C16 pad 2: (no net) -> GND
- C17 pad 1: (no net) -> VDD35
- C17 pad 2: (no net) -> GND
- C18 pad 1: (no net) -> Net-(RA1B-R2.1)
- C18 pad 2: (no net) -> GND
- C19 pad 1: (no net) -> Net-(RA1A-R1.1)
- C19 pad 2: (no net) -> GND
- C2 pad 1: (no net) -> /CPU/LCD/U3-VDD
- C2 pad 2: (no net) -> GND
- C20 pad 1: (no net) -> Net-(RA1C-R3.1)
- C20 pad 2: (no net) -> GND
- C22 pad 1: CSS3 -> /C_SS3
- C22 pad 2: (no net) -> GND
- C23 pad 1: CSS5 -> /C_SS5
- C23 pad 2: (no net) -> GND
- C24 pad 1: (no net) -> /VIN
- C24 pad 2: VIN -> GND
- C25 pad 1: (no net) -> /C_SCP
- C25 pad 2: (no net) -> GND
- C26 pad 1: (no net) -> VDD3
- C26 pad 2: /VDD3 -> GND
- C27 pad 1: (no net) -> VDD2
- C27 pad 2: (no net) -> GND
- C28 pad 1: (no net) -> VDD13
- C28 pad 2: (no net) -> /CPU/LCD/Q1B
- C30 pad 1: (no net) -> GND
- C30 pad 2: (no net) -> /~{RESET}
- C32 pad 1: /LCD-VSS -> /CPU/LCD/P2-VCC
- C32 pad 2: /LCD-VCC -> VDD-15
- C33 pad 1: /LCD-VEE -> /CPU/LCD/P2-VEE
- C33 pad 2: (no net) -> /CPU/LCD/U5-3
- C34 pad 1: (no net) -> VDD3
- C34 pad 2: (no net) -> GND
- C35 pad 1: (no net) -> VDD13
- C35 pad 2: (no net) -> GND
- C36 pad 1: (no net) -> VDD-15
- C36 pad 2: (no net) -> GND
- C37 pad 1: (no net) -> /VOUT3
- C37 pad 2: (no net) -> /REG_EXT
- C38 pad 1: (no net) -> Net-(U6-BC)
- C38 pad 2: (no net) -> GND
- C39 pad 1: (no net) -> Net-(U6-VREF)
- C39 pad 2: (no net) -> GND
- C40 pad 1: (no net) -> /DA1-AC
- C40 pad 2: (no net) -> /T1-6
- C41 pad 1: (no net) -> /DA2-AC
- C41 pad 2: (no net) -> /T1-6
- C43 pad 1: (no net) -> VCC
- C43 pad 2: (no net) -> GND
- C44 pad 1: (no net) -> VDD3
- C44 pad 2: /VDD3 -> GND
- C45 pad 1: (no net) -> /CPU/U6-LOUT
- C45 pad 2: (no net) -> GND
- C46 pad 1: (no net) -> /CPU/U6-ROUT
- C46 pad 2: (no net) -> GND
- C47 pad 1: (no net) -> /CPU/SP
- C47 pad 2: (no net) -> GND
- C48 pad 1: (no net) -> /CPU/FL
- C48 pad 2: (no net) -> /CPU/FL2
- C5 pad 1: /VCC3 -> VDD3
- C50 pad 2: (no net) -> GND
- C51 pad 2: (no net) -> GND
- C52 pad 1: /VDD2 -> VDD2
- C52 pad 2: (no net) -> GND
- C53 pad 1: /VDD2 -> VDD2
- C53 pad 2: (no net) -> GND
- C54 pad 1: (no net) -> /CPU/LCD/U5-3
- C54 pad 2: /VCOM -> /CPU/LCD/VCOM
- C55 pad 1: (no net) -> /VOUT3
- C55 pad 2: (no net) -> GND
- C56 pad 1: /VDD5 -> VDD5
- C56 pad 2: (no net) -> GND
- C57 pad 1: (no net) -> /Q10B
- C57 pad 2: (no net) -> /VSHD
- C58 pad 1: LCD-VDD -> /CPU/LCD/P2-VDD
- C58 pad 2: (no net) -> GND
- C59 pad 1: (no net) -> /CPU/VOL
- C59 pad 2: (no net) -> GND
- C6 pad 1: /VDD35 -> VDD35
- C61 pad 1: (no net) -> /CPU/Q11B
- C61 pad 2: (no net) -> VDD3
- C62 pad 1: /UP -> GND
- C62 pad 2: (no net) -> /CPU/TP6
- C63 pad 1: /R -> GND
- C63 pad 2: (no net) -> /CPU/TP8
- C64 pad 1: (no net) -> GND
- C64 pad 2: (no net) -> /CPU/TP9
- C7 pad 1: /VDD35 -> VDD35
- C8 pad 1: /VDD2 -> VDD2
- C8 pad 2: (no net) -> GND
- C9 pad 1: (no net) -> /CPU/FR2
- C9 pad 2: (no net) -> GND
- CL1 pad 1: /FIQ -> /CPU/FIQ
- CL1 pad 2: /FIQ -> VDD3
- D1 pad 1: (no net) -> /Q9C
- D1 pad 2: (no net) -> /D1A
- D2 pad 2: (no net) -> /D2A
- D2 pad 3: (no net) -> /VOUT5
- D3 pad 2: (no net) -> /D3A
- D3 pad 3: (no net) -> /VOUT3
- D4 pad 1: LCD-VDD -> /CPU/LCD/P2-VDD
- D4 pad 2: (no net) -> GND
- DA1 pad 1: (no net) -> GND
- DA1 pad 2: (no net) -> /DA1-C
- DA1 pad 3: (no net) -> /DA1-AC
- DA2 pad 1: (no net) -> /DA2-A
- DA2 pad 2: (no net) -> GND
- DA2 pad 3: (no net) -> /DA2-AC
- DL1 pad 1: (no net) -> /D1A
- DL1 pad 2: (no net) -> /DL1A
- DL2 pad 1: (no net) -> /DL2K
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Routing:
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- added copper zone on B.Cu, net /BT+
- added copper zone on F.Cu, net /CPU/A_{0}
- added copper zone on F.Cu, net /CPU/A_{10}
- added copper zone on F.Cu, net /CPU/A_{11}
- added copper zone on F.Cu, net /CPU/A_{12}
- added copper zone on F.Cu, net /CPU/A_{13}
- added copper zone on F.Cu, net /CPU/A_{14}
- added copper zone on F.Cu, net /CPU/A_{15}
- added copper zone on F.Cu, net /CPU/A_{1}
- added copper zone on F.Cu, net /CPU/A_{2}
- added copper zone on F.Cu, net /CPU/A_{3}
- added copper zone on F.Cu, net /CPU/A_{4}
- added copper zone on F.Cu, net /CPU/A_{5}
- added copper zone on F.Cu, net /CPU/A_{6}
- added copper zone on F.Cu, net /CPU/A_{7}
- added copper zone on F.Cu, net /CPU/A_{9}
- added copper zone on F.Cu, net /CPU/D_{0}
- added copper zone on F.Cu, net /CPU/D_{1}
- added copper zone on F.Cu, net /CPU/D_{2}
- added copper zone on F.Cu, net /CPU/D_{3}
- added copper zone on F.Cu, net /CPU/D_{4}
- added copper zone on F.Cu, net /CPU/D_{5}
- added copper zone on F.Cu, net /CPU/D_{6}
- added copper zone on F.Cu, net /CPU/D_{7}
- added copper zone on B.Cu, net /CPU/IN35
- added copper zone on F.Cu, net /CPU/IRQ
- added copper zone on B.Cu, net /CPU/LGND
- added copper zone on F.Cu, net /CPU/LGND
- added copper zone on F.Cu, net /CPU/PHI
- added copper zone on F.Cu, net /CPU/RES
- added copper zone on F.Cu, net /CPU/TP3
- added copper zone on F.Cu, net /CPU/TP4
- added copper zone on F.Cu, net /CPU/TP6
- added copper zone on F.Cu, net /CPU/TP7
- added copper zone on B.Cu, net /CPU/VR2-3
- added copper zone on F.Cu, net /CPU/VR2-3
- added copper zone on F.Cu, net /CPU/~{CS}
- added copper zone on F.Cu, net /CPU/~{RD}
- added copper zone on F.Cu, net /CPU/~{WR}
- added copper zone on B.Cu, net /D2A
- added copper zone on F.Cu, net /D2A
- added copper zone on B.Cu, net /D3A
- added copper zone on F.Cu, net /D3A
- added copper zone on B.Cu, net /DA1-AC
- added copper zone on B.Cu, net /SW1-2
- added copper zone on B.Cu, net /T1-6
- added copper zone on B.Cu, net /VOUT3
- added copper zone on F.Cu, net /VOUT3
- added copper zone on B.Cu, net /VOUT5
- added copper zone on B.Cu, net VCC
- added copper zone on B.Cu, net VDD-15
- added copper zone on F.Cu, net VDD-15
- added copper zone on B.Cu, net VDD13
- added copper zone on F.Cu, net VDD13
- added copper zone on B.Cu, net VDD2
- added copper zone on B.Cu, net VDD3
- added copper zone on F.Cu, net VDD3
- added copper zone on B.Cu, net VDD35
- added copper zone on F.Cu, net VDD35
- added copper zone on B.Cu, net VDD5
- added copper zone on F.Cu, net VDD5
- removed copper zone on B.Cu, net (none)
- removed copper zone on F.Cu, net (none)
- removed copper zone on B.Cu, net /VDD2
- removed copper zone on B.Cu, net /VDD3
- removed copper zone on F.Cu, net /VDD3
- removed copper zone on F.Cu, net /VDD35
- removed copper zone on F.Cu, net /VDD5
- removed copper zone on F.Cu, net D3A
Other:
- outline, holes or cut-outs redrawn
- board text added: "'26"
- board text added: "1"
- board text added: "10"
- board text added: "102"
- board text added: "108"
- board text added: "11"
- board text added: "12"
- board text added: "128"
- board text added: "13"
- board text added: "14"
- board text added: "15"
- board text added: "16"
- board text added: "17"
- board text added: "18"
- board text added: "19"
- board text added: "2"
- board text added: "20"
- board text added: "2026"
- board text added: "21"
- board text added: "22"
- board text added: "23"
- board text added: "24"
- board text added: "25"
- board text added: "26"
- board text added: "27"
- board text added: "28"
- board text added: "29"
- board text added: "3"
- board text added: "3-VDD"
- board text added: "30"
- board text added: "31"
- board text added: "32"
- board text added: "38"
- board text added: "39"
- board text added: "4"
- board text added: "40"
- board text added: "5"
- board text added: "6"
- board text added: "64"
- board text added: "7"
- board text added: "8"
- board text added: "9"
- board text added: "A"
- board text added: "A0"
- board text added: "A10"
- board text added: "A12"
- board text added: "A14"
- board text added: "A2"
- board text added: "A4"
- board text added: "A6"
- board text added: "A8"
- board text added: "AGB-AMP"
- board text added: "AGB-CPU"
- board text added: "AGB-REG"
- board text added: "AGB-SRAM"
- board text added: "B"
- board text added: "BT+"
- board text added: "BT-"
- board text added: "C"
- board text added: "C1"
- board text added: "C2"
- board text added: "CPU-01"
- board text added: "CSCP"
- board text added: "CSS3"
- board text added: "CSS5"
- board text added: "D0"
- board text added: "D2"
- board text added: "D4"
- board text added: "D6"
- board text added: "DOWN"
- board text added: "GND"
- board text added: "LEFT"
- board text added: "OAGB-"
- board text added: "OFF"
- board text added: "ON"
- board text added: "P1"
- board text added: "P3"
- board text added: "P4"
- board text added: "RD"
- board text added: "REGEXT"
- board text added: "RESET"
- board text added: "RIGHT"
- board text added: "S1"
- board text added: "S2"
- board text added: "SELECT"
- board text added: "SO1"
- board text added: "SO2"
- board text added: "SP1"
- board text added: "START"
- board text added: "SW2"
- board text added: "SW3"
- board text added: "U"
- board text added: "U1"
- board text added: "U2"
- board text added: "U3"
- board text added: "U4"
- board text added: "U6"
- board text added: "UP"
- board text removed: "Redherring32 2023"
